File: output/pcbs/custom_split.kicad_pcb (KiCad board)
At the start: 2 copper layers, 135.1 x 84 mm, 23 parts

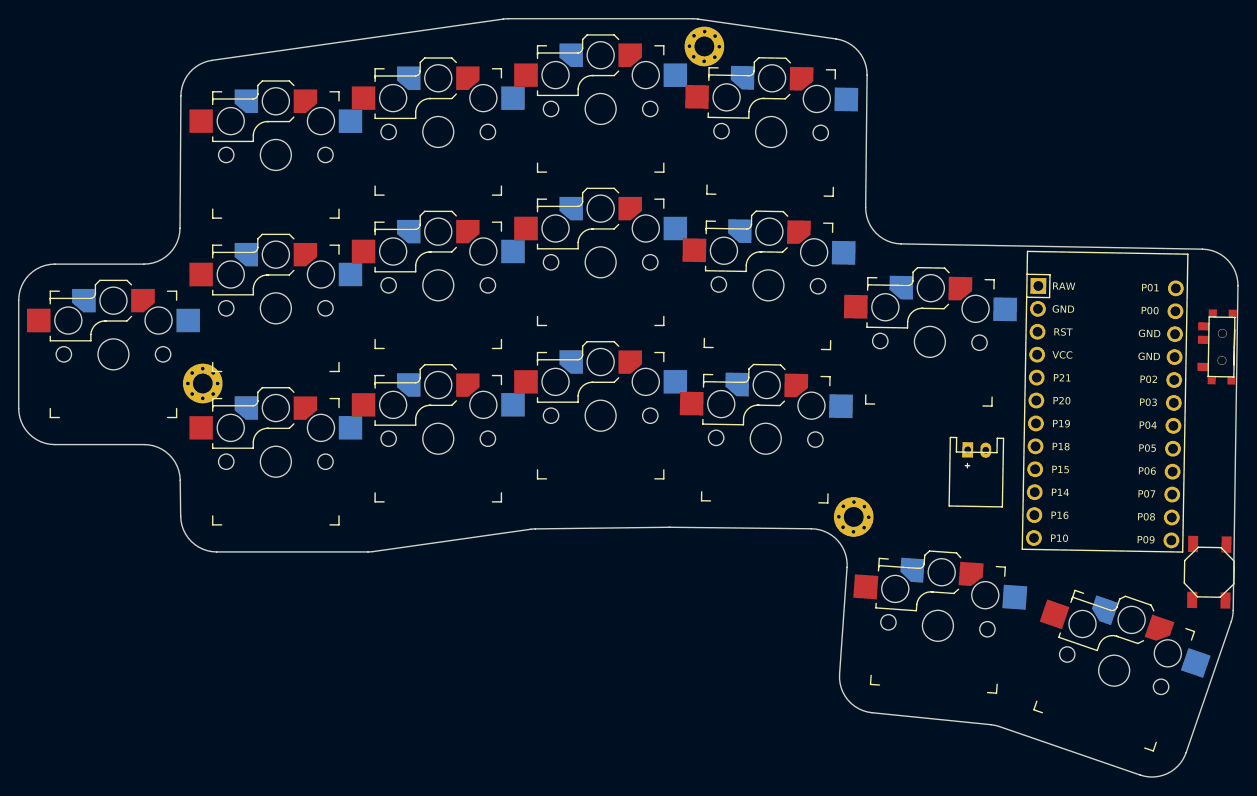
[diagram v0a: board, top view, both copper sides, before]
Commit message: forgot to save the bp
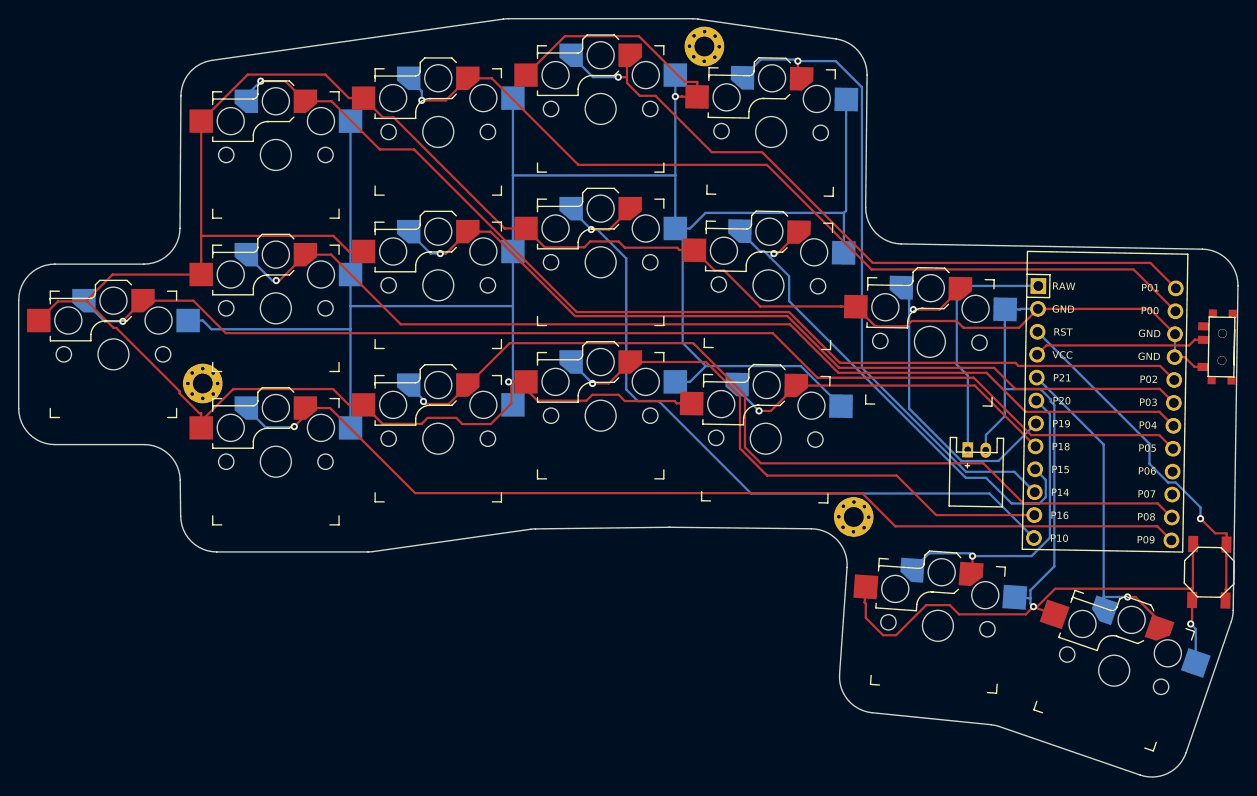
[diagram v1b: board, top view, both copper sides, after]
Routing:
- net GND: track 0.00 -> 622.0 mm, vias 0 -> 4
- net P5: track 0.00 -> 129.4 mm, vias 0 -> 1
- net P2: track 0.00 -> 117.9 mm, vias 0 -> 1
- net P4: track 0.00 -> 113.0 mm, vias 0 -> 1
- net P9: track 0.00 -> 110.9 mm, vias 0 -> 1
- net P8: track 0.00 -> 99.8 mm, vias 0 -> 1
- net P0: track 0.00 -> 98.3 mm, vias 0 -> 1
- net P3: track 0.00 -> 94.7 mm, vias 0 -> 1
- net P1: track 0.00 -> 80.7 mm, vias 0 -> 1
- net P10: track 0.00 -> 80.2 mm, vias 0 -> 1
- net P14: track 0.00 -> 73.4 mm, vias 0 -> 1
- net P16: track 0.00 -> 63.7 mm, vias 0 -> 1
- net P15: track 0.00 -> 56.2 mm, vias 0 -> 1
- net RST: track 0.00 -> 39.7 mm, vias 0 -> 1
- net P19: track 0.00 -> 38.6 mm, vias 0 -> 1
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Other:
- net class Default removed
